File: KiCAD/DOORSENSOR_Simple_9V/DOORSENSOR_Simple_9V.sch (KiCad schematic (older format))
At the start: 11 parts, among them J1 9V, Q1 NTR4003NT1G, SW1 Trigger, SW2 Open/Close, SW3 Pairing, U1 AMS1117-3.3, U2 ESP-12F

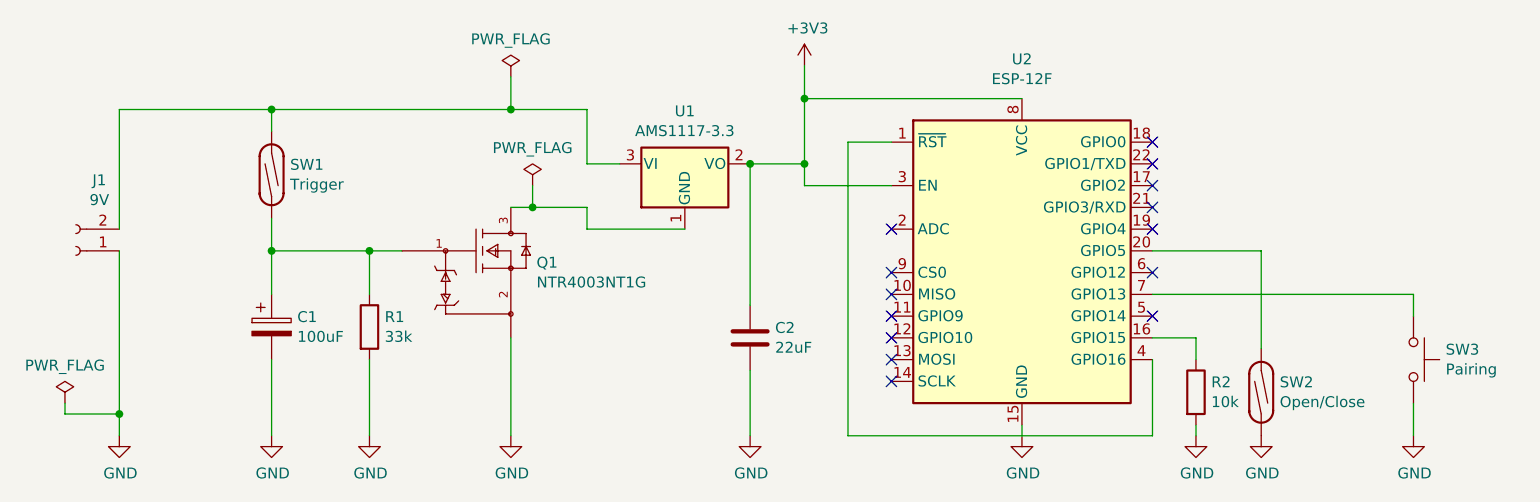
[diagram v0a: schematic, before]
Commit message: Update
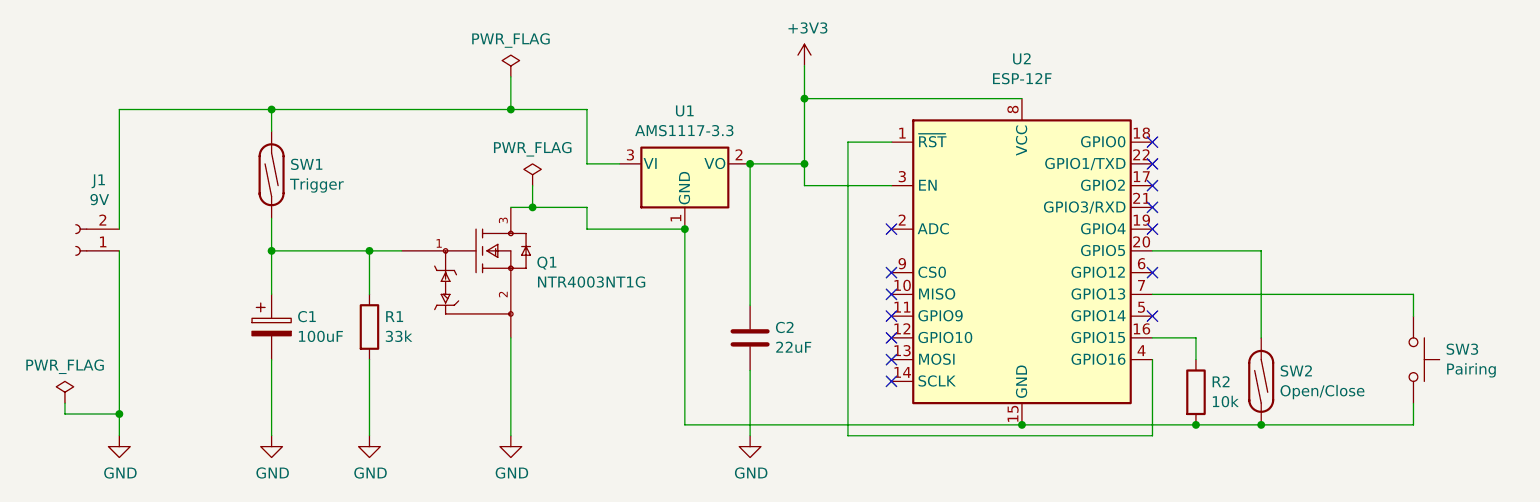
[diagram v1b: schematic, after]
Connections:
- net GND: no longer R2.2, SW2.2, SW3.2, U2.15 (GND)
- net at Q1.3 (D), U1.1 (GND): now also R2.2, SW2.2, SW3.2, U2.15 (GND)
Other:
- moved on the sheet: SW2
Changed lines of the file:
@@
 $EndComp
-$Comp
-L power:GND #PWR07
-U 1 1 6077856C
-P 5150 3100
-F 0 "#PWR07" H 5150 2850 50  0001 C CNN
-F 1 "GND" H 5155 2927 50  0000 C CNN
-F 2 "" H 5150 3100 50  0001 C CNN
-F 3 "" H 5150 3100 50  0001 C CNN
-	1    5150 3100
-	1    0    0    -1
-$EndComp
-Wire Wire Line
-	5150 3050 5150 3100
 $Comp
 L Switch:SW_Reed SW2
 U 1 1 607790E4
-P 6250 2900
-F 0 "SW2" V 6204 2985 50  0000 L CNN
-F 1 "Open/Close" V 6295 2985 50  0000 L CNN
-F 2 "SHRDZM:Magnetic Reed Relay" H 6250 2900 50  0001 C CNN
-F 3 "~" H 6250 2900 50  0001 C CNN
-	1    6250 2900
+P 6250 2850
+F 0 "SW2" V 6204 2935 50  0000 L CNN
+F 1 "Open/Close" V 6295 2935 50  0000 L CNN
+F 2 "SHRDZM:Magnetic Reed Relay" H 6250 2850 50  0001 C CNN
+F 3 "~" H 6250 2850 50  0001 C CNN
+	1    6250 2850
 	0    1    1    0
-$EndComp
-$Comp
-L power:GND #PWR09
-U 1 1 6077A1D1
-P 6250 3100
-F 0 "#PWR09" H 6250 2850 50  0001 C CNN
-F 1 "GND" H 6255 2927 50  0000 C CNN
-F 2 "" H 6250 3100 50  0001 C CNN
-F 3 "" H 6250 3100 50  0001 C CNN
-	1    6250 3100
-	1    0    0    -1
 $EndComp
 $Comp
@@
 Wire Wire Line
 	5950 2650 5950 2750
-$Comp
-L power:GND #PWR08
-U 1 1 6077B6AB
-P 5950 3100
-F 0 "#PWR08" H 5950 2850 50  0001 C CNN
-F 1 "GND" H 5955 2927 50  0000 C CNN
-F 2 "" H 5950 3100 50  0001 C CNN
-F 3 "" H 5950 3100 50  0001 C CNN
-	1    5950 3100
-	1    0    0    -1
-$EndComp
-Wire Wire Line
-	5950 3050 5950 3100
 $Comp
 L eec:NTR4003NT1G Q1
@@
 	6250 2250 5750 2250
 Wire Wire Line
-	6250 2250 6250 2700
-Wire Wire Line
 	5750 2750 5750 3100
 Wire Wire Line
@@
 Wire Wire Line
 	5750 2450 6950 2450
-$Comp
-L power:GND #PWR010
-U 1 1 60793010
-P 6950 3100
-F 0 "#PWR010" H 6950 2850 50  0001 C CNN
-F 1 "GND" H 6955 2927 50  0000 C CNN
-F 2 "" H 6950 3100 50  0001 C CNN
-F 3 "" H 6950 3100 50  0001 C CNN
-	1    6950 3100
-	1    0    0    -1
-$EndComp
 Wire Wire Line
 	6950 2450 6950 2550
-Wire Wire Line
-	6950 2950 6950 3100
 NoConn ~ 4550 2850
 NoConn ~ 4550 2750
@@
 Wire Wire Line
 	1000 1600 1000 2150
+Wire Wire Line
+	5150 3050 3600 3050
+Wire Wire Line
+	3600 3050 3600 2150
+Connection ~ 3600 2150
+Wire Wire Line
+	5950 3050 5150 3050
+Connection ~ 5150 3050
+Wire Wire Line
+	6250 3050 5950 3050
+Connection ~ 5950 3050
+Wire Wire Line
+	6950 2950 6950 3050
+Wire Wire Line
+	6950 3050 6250 3050
+Connection ~ 6250 3050
+Wire Wire Line
+	6250 2250 6250 2650
 $EndSCHEMATC
